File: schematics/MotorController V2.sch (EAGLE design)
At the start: 51 parts, among them IC1 7805, Q1 BC307

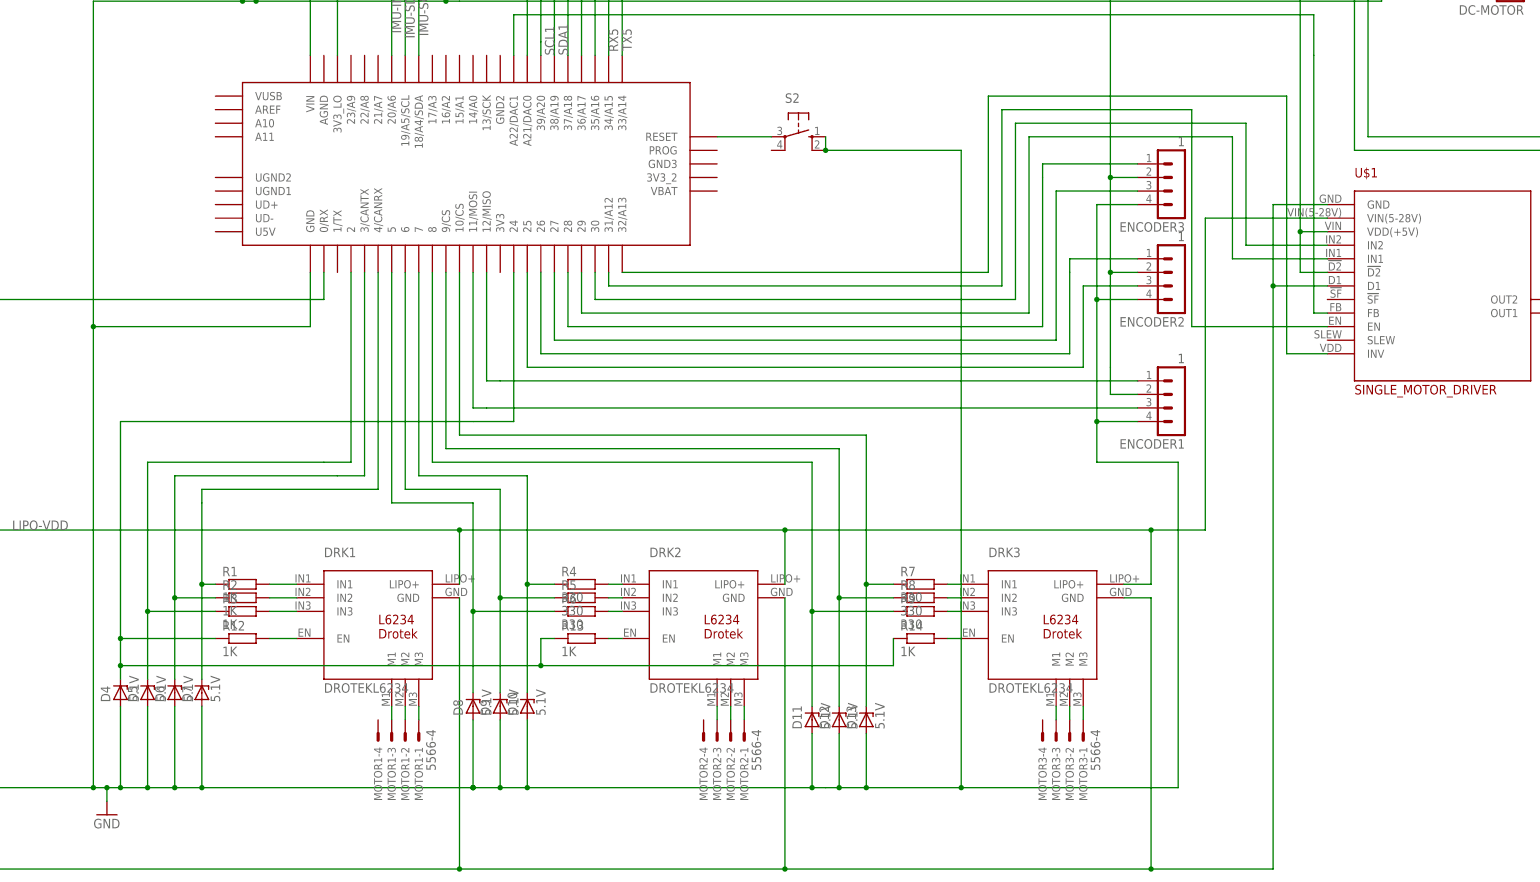
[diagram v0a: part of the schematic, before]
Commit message: no message
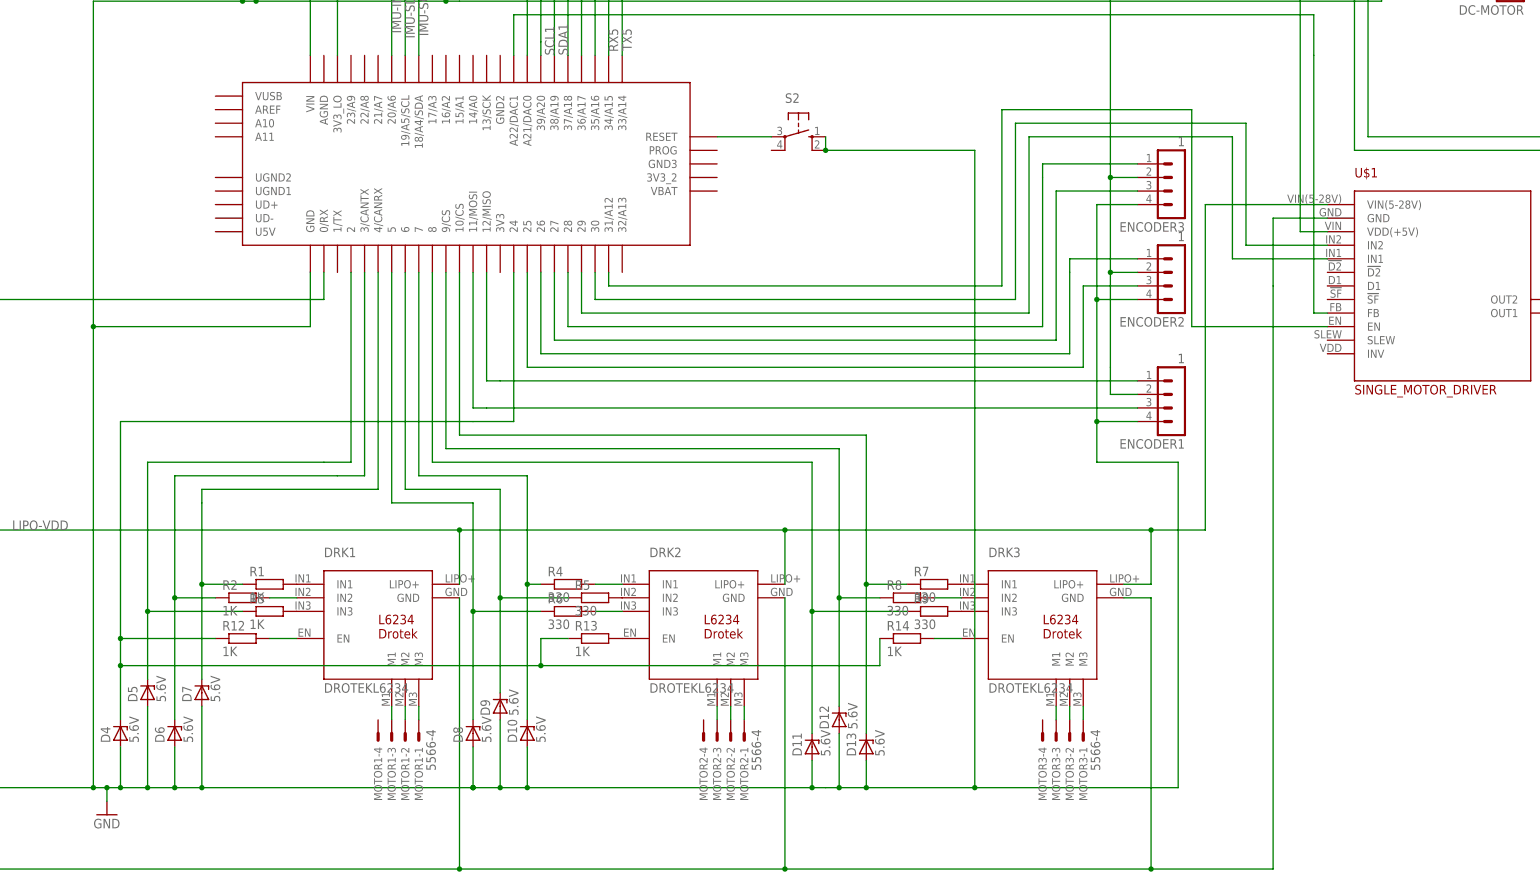
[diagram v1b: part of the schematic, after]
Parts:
- D10, D11, D12, D13, D4, D5, D6, D7, D8, D9: value 5.1V -> 5.6V
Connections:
- removed net N$41: PRJ1.32/A13, U$1.INV
- net LIPO-GND: no longer U$1.D1
- net VCC: no longer U$1.!D2
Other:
- moved on the sheet: D10, D11, D13, D4, D6, D8, R1, R13, R14, R3, R4, R5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
